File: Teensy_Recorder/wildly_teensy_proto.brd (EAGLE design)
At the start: 55.4 x 78.2 mm, 34 parts, among them J1 61300211121, J2 61300311121, J3 61300311121, T1 BC847BLT1G, T2 BC847BLT1G, T3 BC847BLT1G

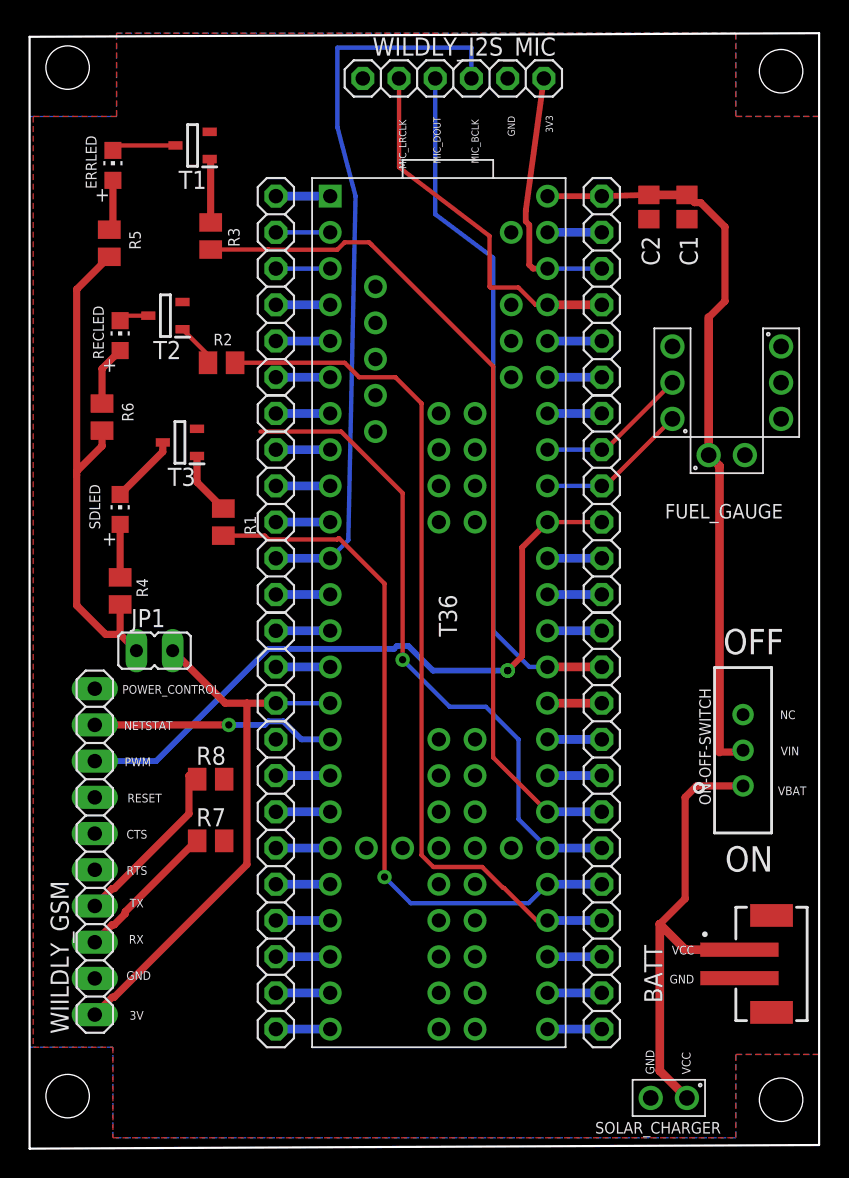
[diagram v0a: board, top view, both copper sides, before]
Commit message: Add GSM signals, rerouting for space efficiency and minor changes for fabrication
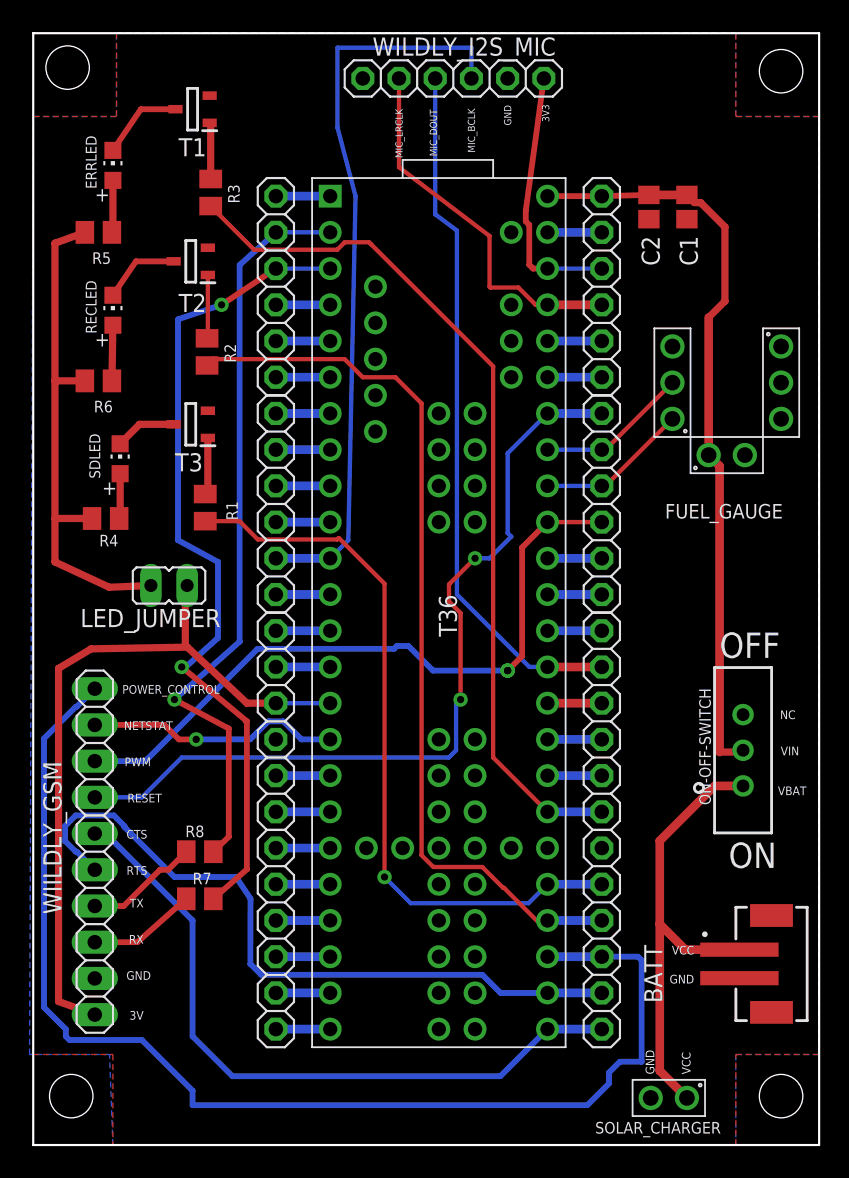
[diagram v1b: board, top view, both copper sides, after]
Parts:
- removed JP1: (no value), jumper:JP1
- added LED_JUMPER: (no value), jumper:JP1
- moved R4 5.18 mm to (10.7, 43.4), turned to 180 degrees
- moved R8 5.14 mm to (17.3, 20.1)
- moved T2 4.20 mm to (16.6, 61.5)
- moved R7 4.13 mm to (17.3, 16.8)
- moved SDLED 3.56 mm to (11.7, 47.6)
- moved R3 3.05 mm to (18.0, 66.3)
- moved R6 2.55 mm to (10.2, 53.1), turned to 180 degrees
- moved T1 2.54 mm to (16.8, 72.1)
- moved RECLED 1.85 mm to (11.2, 58.0)
- moved R1 1.63 mm to (17.7, 44.2)
- moved T3 1.48 mm to (16.6, 50.0)
- moved R2 1.27 mm to (17.8, 55.1), turned to 90 degrees
- moved R5 1.08 mm to (10.2, 63.5), turned to 180 degrees
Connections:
- removed net POWER_CNTROL: WIILDLY_GSM.10
- removed net RESET_OF_GSM: WIILDLY_GSM.7
- net +3V3: now also LED_JUMPER.1; no longer JP1.1
- net 3V3: now also LED_JUMPER.2; no longer JP1.2
- net NETSTATLED: no longer U$1.38
- net POWER_CONTROL: now also WIILDLY_GSM.10
- net RESET_GSM: now also WIILDLY_GSM.7
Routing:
- net POWER_CONTROL: track 3.81 -> 85.0 mm
- net RX_OF_GSM: track 3.81 -> 58.6 mm, vias 0 -> 2
- net RESET_GSM: track 3.81 -> 58.3 mm, vias 0 -> 2
- net TX_OF_GSM: track 3.81 -> 53.2 mm, vias 0 -> 1
- net RTS_OF_GSM: track 3.81 -> 50.0 mm
- net NETSTATLED: track 46.2 -> 0.00 mm, vias 1 -> 0
- net CTS_OF_GSM: track 3.81 -> 48.7 mm
- net 3V3: track 58.4 -> 71.0 mm
- net N$12: track 12.6 -> 7.99 mm
- net N$2: track 2.12 -> 5.52 mm
- net N$10: track 10.2 -> 7.57 mm
- net RECLED: track 60.5 -> 62.7 mm
- net SDLED: track 49.9 -> 51.6 mm
- net N$4: track 4.53 -> 5.92 mm
- net N$3: track 3.09 -> 4.47 mm
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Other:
- board size 55.4 x 78.2 mm -> 55.1 x 78 mm
